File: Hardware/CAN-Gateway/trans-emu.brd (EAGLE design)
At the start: 29 x 34 mm, 40 parts, among them IC1 MIC5233-3.3YM5-TR, Q1 PMOSFET, Q2 NMOSFET, U1 STM32F413RGT6, U2 TJA1042HVSON, U3 TJA1042HVSON, U4 TJA1042HVSON, Y1 CRYSTAL-3.2X2.54-PIN

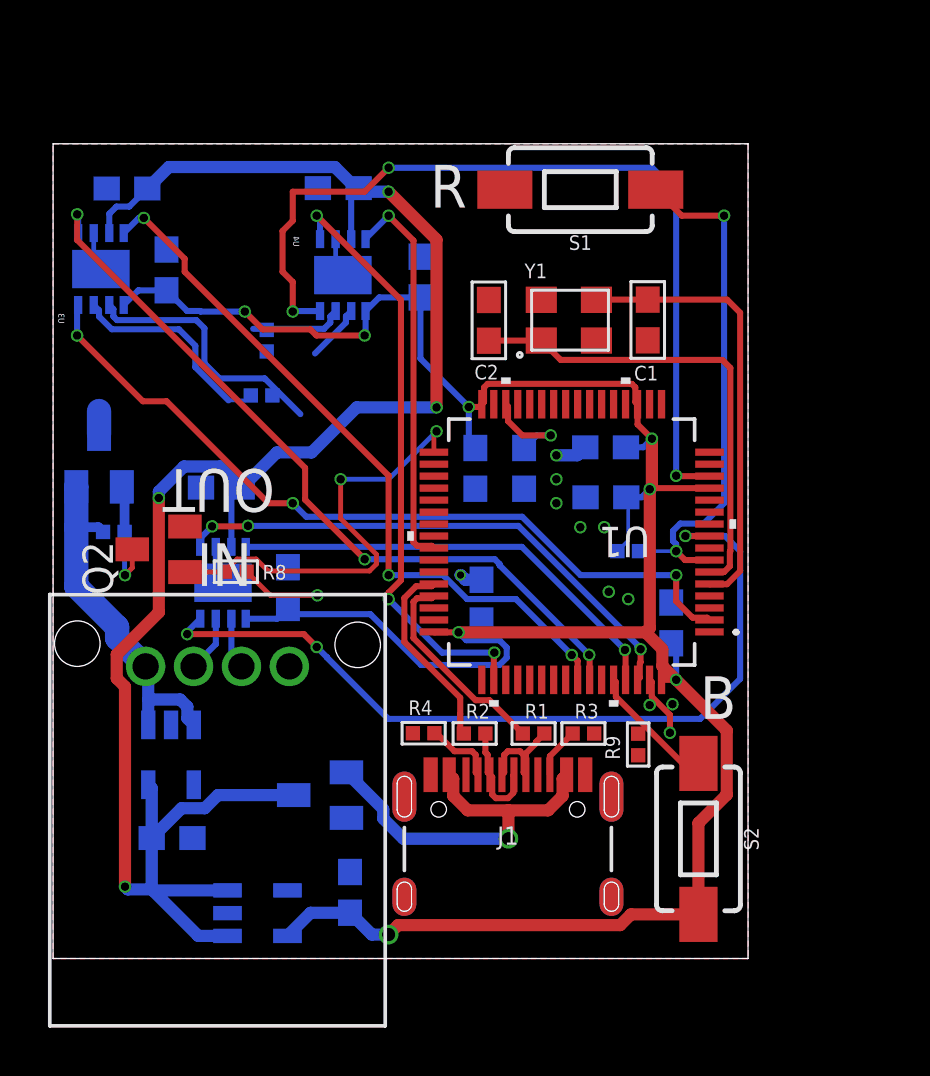
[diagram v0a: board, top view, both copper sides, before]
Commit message: Gateway rev2
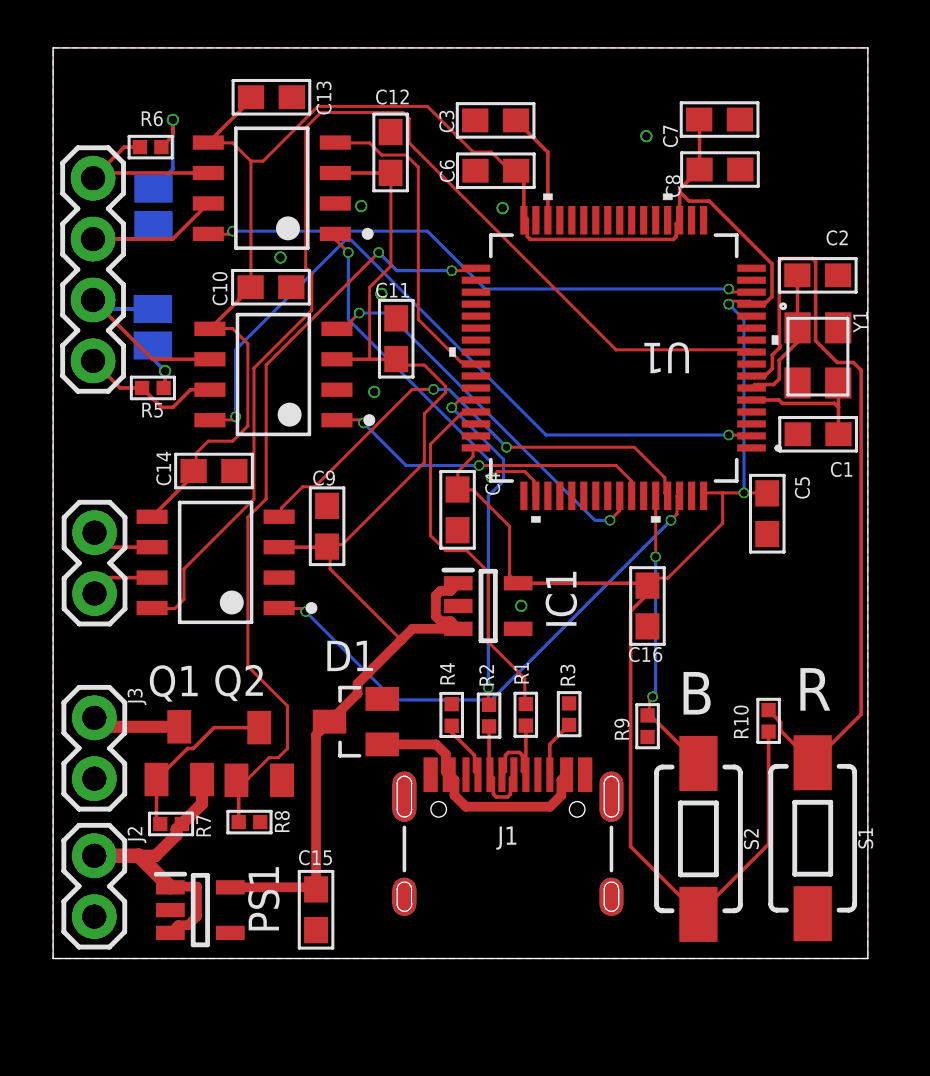
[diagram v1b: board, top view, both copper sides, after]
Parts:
- removed U$1: MINI50-4, interceptor:MINI50
- added J2, J3, J4: (no value), SparkFun-Connectors:1X02
- added J5: (no value), SparkFun-Connectors:1X04
- added SJ1, SJ2: (no value), jumper:SJ
- U2, U3, U4: value TJA1042HVSON -> TJA1042; device comma.ai:HVSON8 -> CM,118:NXP_SEMICONDUCTORS_TJA1042T-3-CM_118_0
- moved S1 28.8 mm to (31.7, 5.02), turned to 270 degrees
- moved C16 17.2 mm to (24.8, 14.7), flipped to the top, turned to 270 degrees
- moved IC1 16.0 mm to (18.2, 14.7), flipped to the top, turned to 0 degrees
- moved C3 14.6 mm to (18.5, 35.0), flipped to the top, turned to 180 degrees
- moved C7 14.5 mm to (27.8, 35.0), flipped to the top
- moved C8 14.5 mm to (27.8, 32.9), flipped to the top
- moved C2 13.9 mm to (31.9, 28.5), turned to 0 degrees
- moved C11 12.9 mm to (14.3, 25.9), flipped to the top, turned to 90 degrees
- moved Q1 12.7 mm to (5.26, 8.57), flipped to the top
- moved Y1 12.6 mm to (32.9, 26.3), turned to 270 degrees
- moved C10 12.6 mm to (9.09, 28.0), flipped to the top, turned to 0 degrees
- moved C6 12.4 mm to (18.5, 32.9), flipped to the top, turned to 180 degrees
- moved R7 12.4 mm to (4.92, 5.61), flipped to the top
- moved R8 10.5 mm to (8.19, 5.69)
- moved C13 9.75 mm to (9.11, 35.9), flipped to the top, turned to 0 degrees
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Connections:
- removed net N$15: Q1.3
- new net 12VOUT: J3.1, Q1.3
- new net CAN1_H: J4.1, U2.7
- new net CAN1_L: J4.2, U2.6
- net 12V: now also J2.1; no longer U$1.4
- net CAN2_H: now also J5.1
- net CAN2_L: now also J5.2, SJ1.1; no longer R5.2
- net CAN3_H: now also J5.3, SJ2.1; no longer R6.1
- net CAN3_L: now also J5.4
- net GND: now also J2.2, J3.2; no longer U$1.1, U2.PAD, U3.PAD, U4.PAD
- net N$12: now also R5.2, SJ1.2; no longer U$1.3, U2.7
- net N$14: now also R6.1, SJ2.2; no longer U$1.2, U2.6
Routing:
- net 5V: track 78.9 -> 53.0 mm, vias 4 -> 0
- net CAN2_TX: track 32.3 -> 14.0 mm, vias 3 -> 2
- net CAN2_RX: track 30.4 -> 16.4 mm, vias 3 -> 2
- net PWRON: track 18.6 -> 32.5 mm
- net N$2: track 19.8 -> 5.96 mm
- net GND: track 13.3 -> 0.00 mm, vias 12 -> 7
- net CAN3_EN: track 36.6 -> 23.8 mm, vias 3 -> 2
- net N$1: track 18.5 -> 5.90 mm
- net CAN1_EN: track 35.0 -> 47.1 mm, vias 3 -> 0
- net N$8: track 21.9 -> 33.1 mm, vias 2 -> 0
- net CAN3_TX: track 25.2 -> 15.6 mm, vias 3 -> 2
- net 3.3V: track 106.6 -> 113.6 mm, vias 8 -> 2
- net N$4: track 8.68 -> 15.5 mm
- net N$3: track 8.16 -> 14.7 mm, vias 0 -> 2
- net N$9: track 5.78 -> 12.3 mm, vias 0 -> 2
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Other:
- board size 29 x 34 mm -> 34 x 38 mm
- board text added: "12V"
- board text added: "12VOUT"
- board text added: "CAN1H"
- board text added: "CAN1L"
- board text added: "CAN2H"
- board text added: "CAN2L"
- board text added: "CAN3H"
- board text added: "CAN3L"
- board text added: "GND"
- board text added: "Ocelot CAN Gateway"
- board text removed: "IN"
- board text removed: "OUT"
- board text removed: "Ocelot CAN Translator"
